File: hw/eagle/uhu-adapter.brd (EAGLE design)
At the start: 46.3 x 28.2 mm, 17 parts, among them IC1 STM32F303CBT

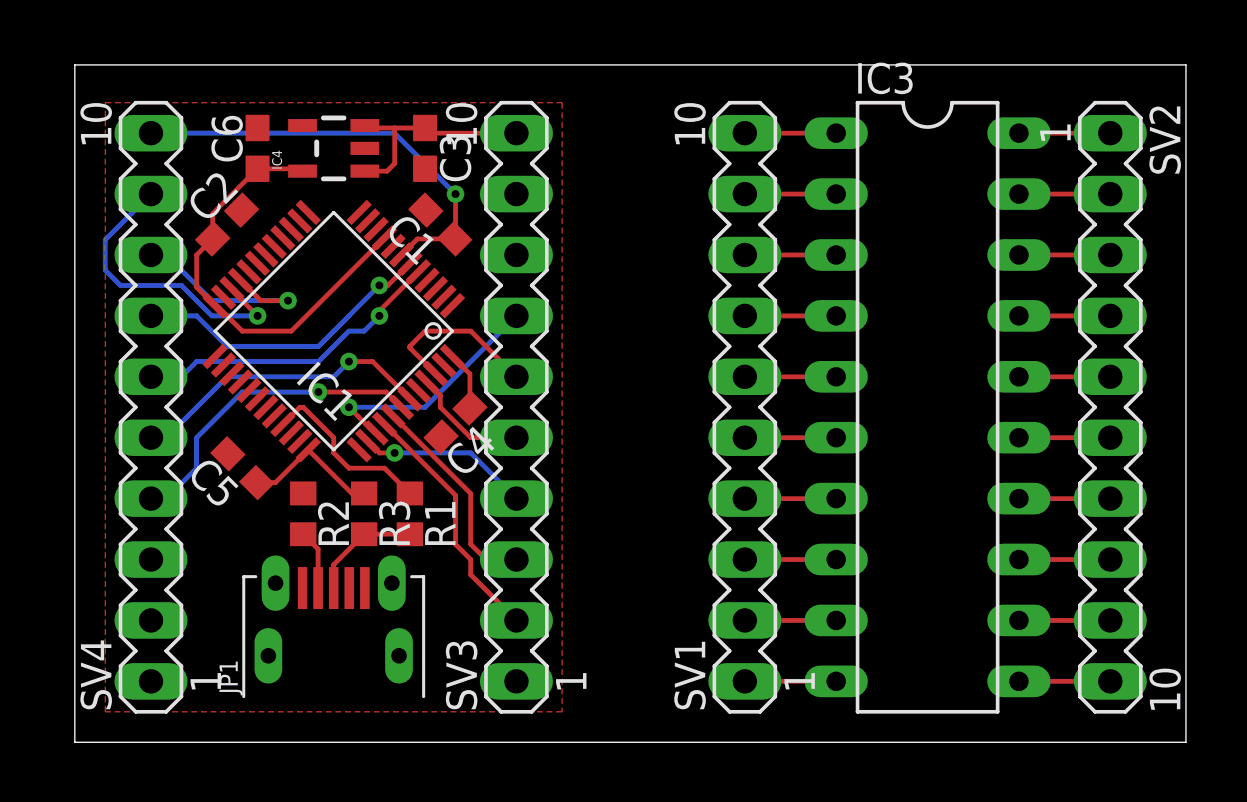
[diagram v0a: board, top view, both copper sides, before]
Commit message: uhu adapter
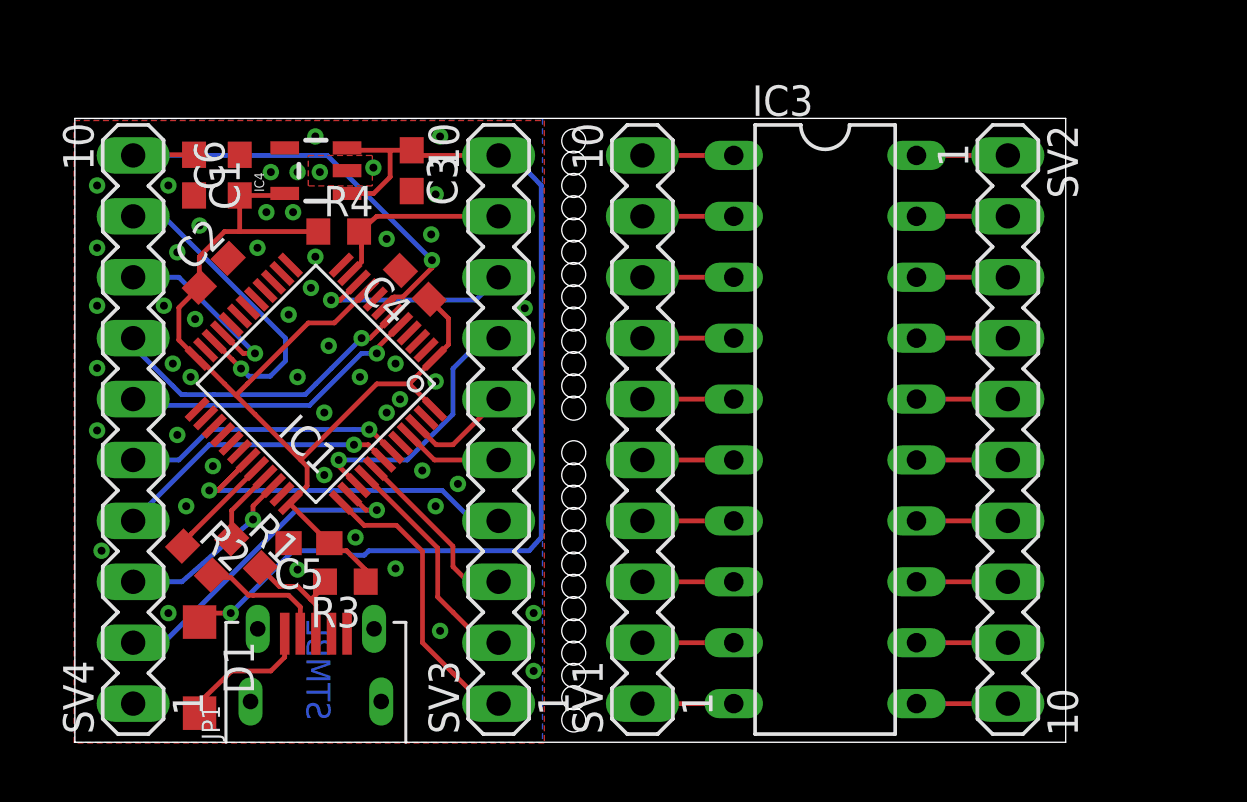
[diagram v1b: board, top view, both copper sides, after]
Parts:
- added D1: (no value), diode:SOD123
- added R4: 10k, rcl:R0603
- C1, C2, C3, C4, C5, C6: value (none) -> 100n
- moved C1 10.5 mm to (4.97, 23.7), turned to 270 degrees
- moved R1 7.02 mm to (7.14, 7.88), turned to 315 degrees
- moved C4 5.98 mm to (14.2, 19.1), turned to 135 degrees
- moved R2 4.84 mm to (5.10, 7.58), turned to 315 degrees
- moved IC3 4.37 mm to (31.3, 13.0)
- moved SV1 4.37 mm to (23.7, 13.0)
- moved SV2 4.37 mm to (38.9, 13.0)
- moved C5 4.18 mm to (9.76, 8.30), turned to 180 degrees
- moved R3 2.94 mm to (11.3, 6.70), turned to 180 degrees
- moved IC1 2.32 mm to (10.1, 14.9)
- moved C2 2.09 mm to (5.79, 19.6)
- moved JP1 2.04 mm to (10.1, 0.00)
- moved C6 1.34 mm to (6.88, 23.7)
- moved IC4 1.19 mm to (10.1, 23.8)
- moved SV4 1.19 mm to (2.43, 13.0)
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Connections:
- removed net IO0: SV4.3
- removed net IO2: SV3.1
- new net 5VUSB: D1.A, JP1.1
- new net N$21: IC1.2
- new net N$22: IC1.3
- new net N$25: IC1.4
- new net SWCLK: IC1.37, SV3.1
- new net SWDIO: IC1.34, SV4.3
- net 3V3: now also R4.1
- net 5V: now also D1.C
- net GND: now also IC1.44
- net IO1: now also IC1.38
- net IO3: now also IC1.10
- net IO4: now also IC1.11, R4.2
- net START: now also IC1.31; no longer IC1.38
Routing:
- net 5V: track 9.31 -> 42.7 mm, vias 0 -> 1
- net 3V3: track 26.4 -> 46.7 mm
- net IO1: track 0.00 -> 13.9 mm, vias 0 -> 1
- net SWCLK: track 0.00 -> 12.3 mm
- net START: track 7.20 -> 16.5 mm
- net IO3: track 0.00 -> 8.82 mm, vias 0 -> 1
- net IO4: track 0.00 -> 8.11 mm
- net SWDIO: track 0.00 -> 7.74 mm, vias 0 -> 1
- net 5VUSB: track 0.00 -> 5.75 mm
- net DM: track 0.00 -> 4.47 mm
- net DP: track 7.45 -> 3.15 mm
- net N$24: track 2.50 -> 5.38 mm
- net EN: track 7.07 -> 4.49 mm
- net NRST: track 18.1 -> 20.2 mm
- net B: track 8.86 -> 7.59 mm
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- added copper zone on layer 16, net GND
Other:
- board size 46.3 x 28.2 mm -> 41.3 x 26 mm
- board text added: "STMBL"
